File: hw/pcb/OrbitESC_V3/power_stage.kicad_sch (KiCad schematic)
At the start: 53 parts, among them U13 TLV9051IDBVR, U14 TLV9051IDBVR, U4 TLV9051IDBVR, U5 DRV8300DRGER

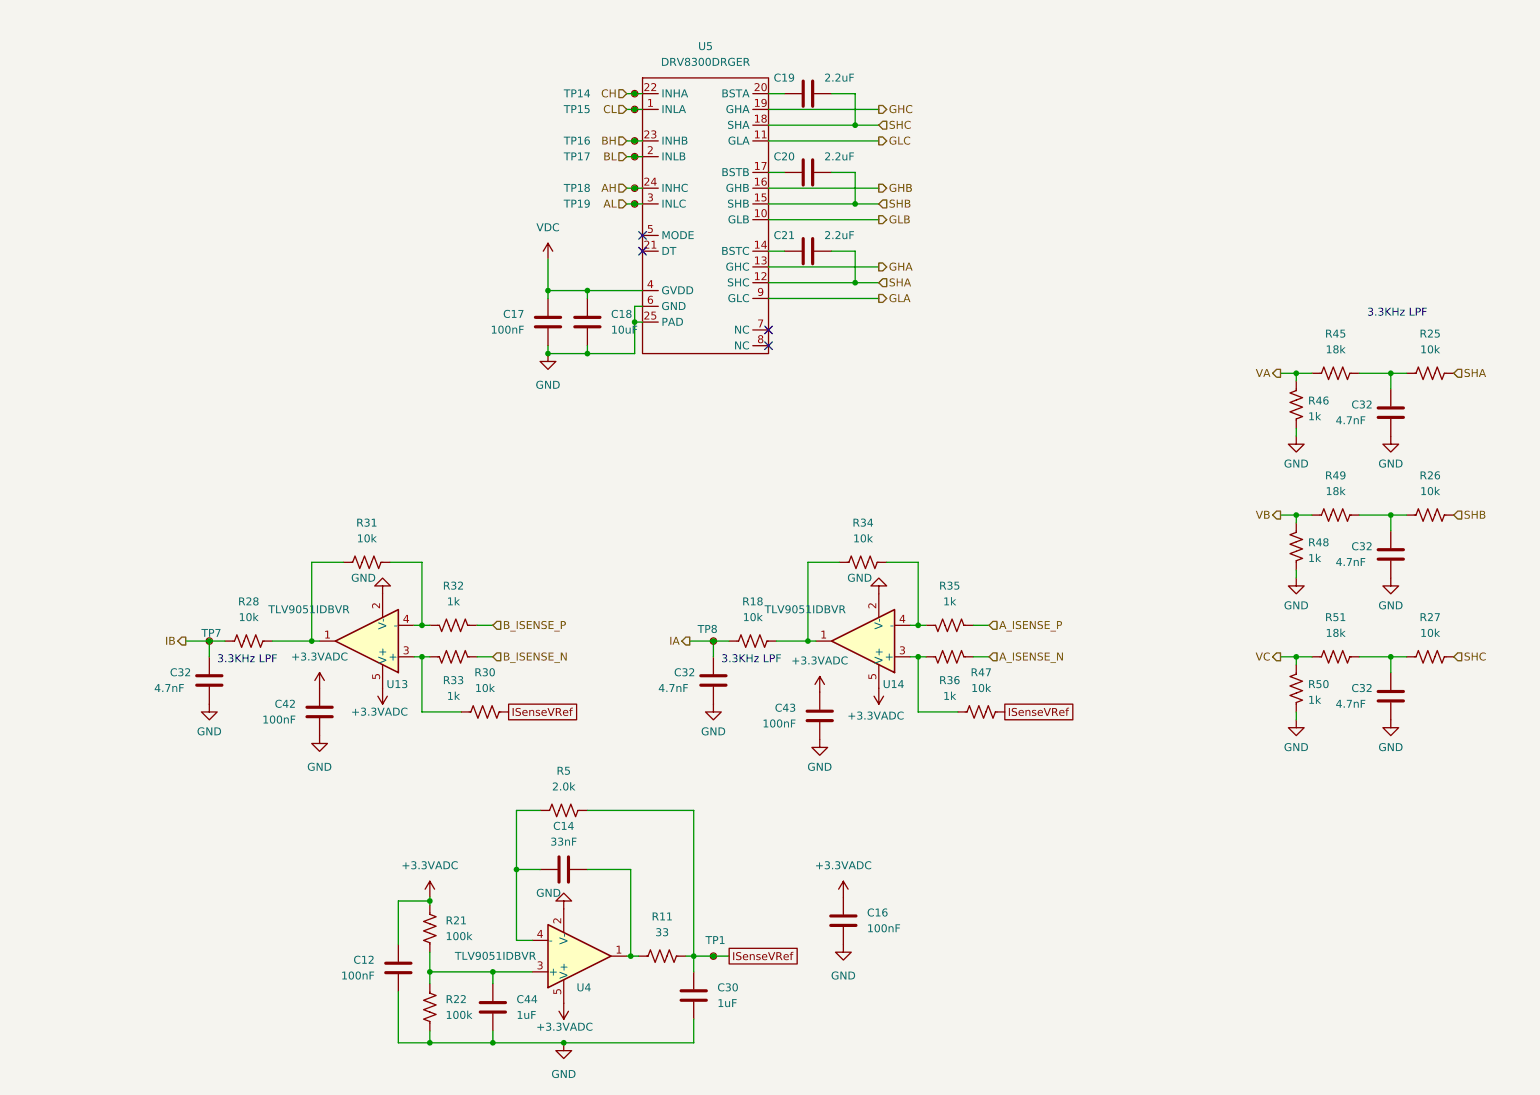
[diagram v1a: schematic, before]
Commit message: PCB work over lunch
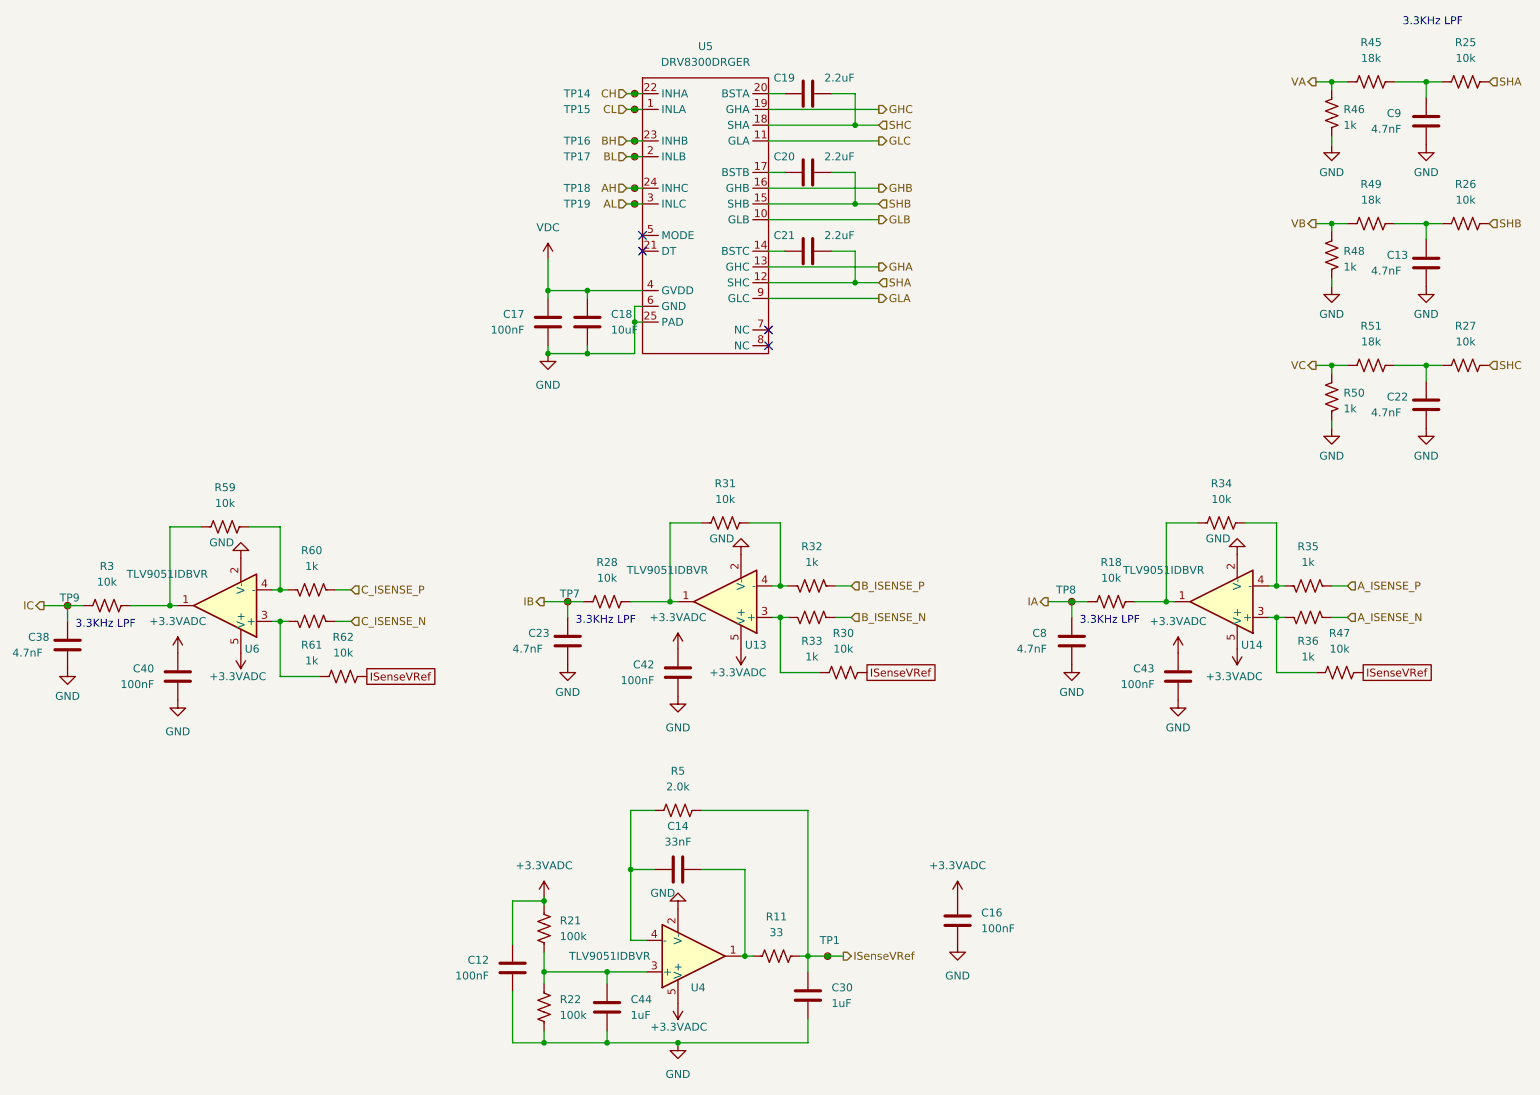
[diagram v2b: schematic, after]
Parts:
- added C38: 4.7nF, Capacitor_SMD:C_0402_1005Metric, symbol Device:C
- added C40: 100nF, Capacitor_SMD:C_0402_1005Metric, symbol Device:C
- added R3, R59, R62: 10k, Resistor_SMD:R_0402_1005Metric, symbol Device:R_US
- added R60, R61: 1k, Resistor_SMD:R_0402_1005Metric, symbol Device:R_US
- added TP9: AH, TestPoint:TestPoint_Pad_D1.0mm, symbol Connector:TestPoint_Small
- added U6: TLV9051IDBVR, Package_TO_SOT_SMD:SOT-23-5, symbol Amplifier_Operational:TLV9001IDCK
- renumbered C32 to C13, C32 to C22, C32 to C23, C32 to C8, C32 to C9
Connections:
- net +3.3VADC: now also C40.1, U6.5 (V+)
- net GND: now also C38.1, C40.2, U6.2 (V-)
- net ISenseVRef: now also R62.2
- new net: R3.2, R59.1, U6.1
- new net: R61.2, R62.1, U6.3 (+)
- new net: R59.2, R60.2, U6.4 (-)
- new net C_ISENSE_N: R61.1
- new net C_ISENSE_P: R60.1
- new net IC: C38.2, R3.1, TP9.1
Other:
- moved on the sheet: C12, C13, C14, C16, C22, C23, C30, C42, C43, C44, C8, C9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
